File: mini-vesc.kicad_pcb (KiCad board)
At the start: 4 copper layers, 65 x 18 mm, 151 parts, among them P1 CONN_1, P10 CONN_01X06, P11 CONN_01X06, P2 CONN_1, P3 CONN_1, P4 CONN_1, P5 CONN_1, P6 CONN_1, P9 CONN_01X06, Q1 NTMFS5C604NLT1G, Q2 NTMFS5C604NLT1G, Q3 NTMFS5C604NLT1G, Q4 NTMFS5C604NLT1G, Q5 NTMFS5C604NLT1G, Q6 NTMFS5C604NLT1G, U1 LM5113, U10 MCP1700, U2 LM5113, U3 LM5113, U4 AD8418, U5 AD8418, U6 AD8418, U7 STM32F40X_LQFP64, U8 LMR16006, U9 MCP1700, X1 ABM3B-8.000MHZ

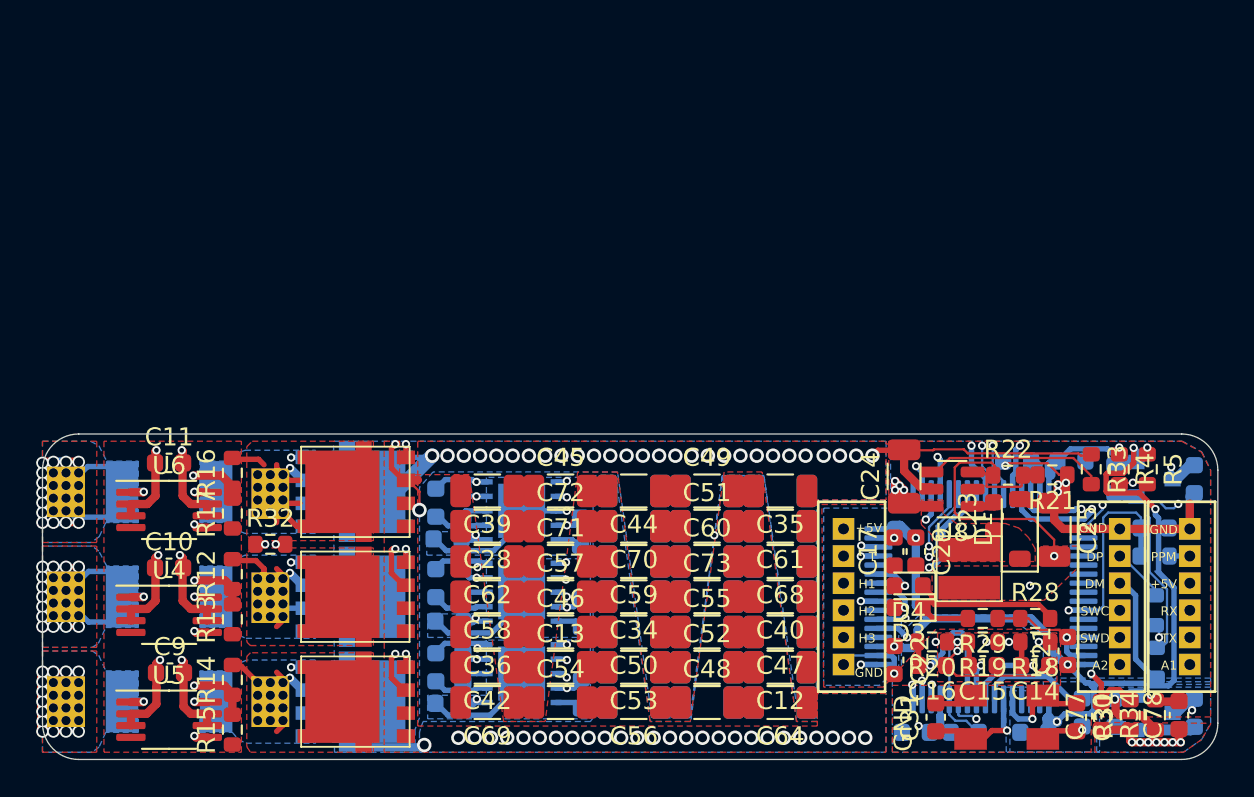
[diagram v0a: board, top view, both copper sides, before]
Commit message: Playing around with routing
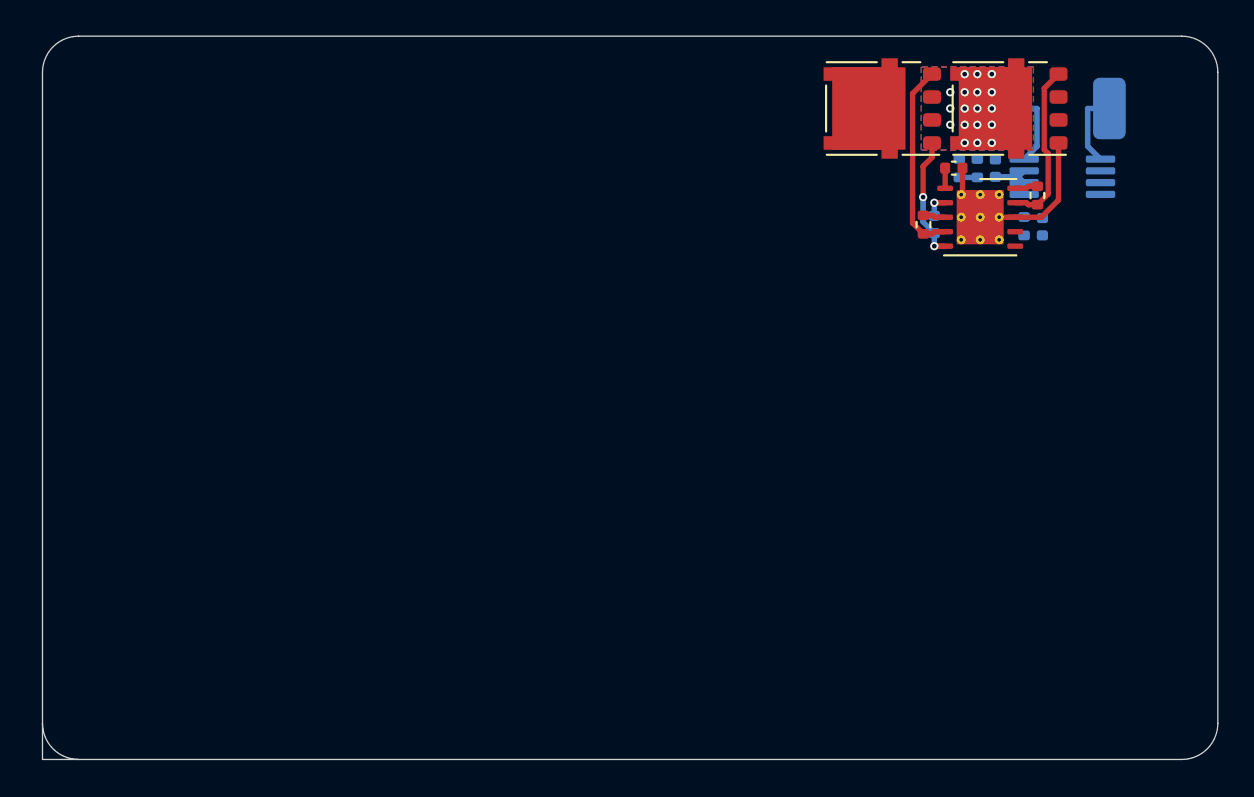
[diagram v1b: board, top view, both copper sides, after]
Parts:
- removed C1, C2, C3: 470n, Capacitor_SMD:C_0603_1608Metric
- removed C10, C11, C17, C18, C6, C7, C77, C78, C8, C86, C87, C88, C89, C9, C90: 2u2, Capacitor_SMD:C_0603_1608Metric
- removed C12, C13, C25, C28, C32, C39, C4, C48, C5, C60, C61, C62, C63, C74, C75, C84, C85: 10u, Capacitor_SMD:C_1206_3216Metric
- removed C14, C15, C16: 4n7, Capacitor_SMD:C_0603_1608Metric
- removed C19, C20, C21, C22, C26, C27, C29, C76: 100n, Capacitor_SMD:C_0603_1608Metric
- removed C23: 220nF, Capacitor_SMD:C_0603_1608Metric
- removed C24: 2u2, Capacitor_SMD:C_1206_3216Metric
- removed C30, C31: 10pF, Capacitor_SMD:C_0603_1608Metric
- removed C33, C34, C35, C36, C37, C38, C40, C41, C42, C43, C44, C45, C46, C47, C49, C50, C51, C52, C53, C54, C55, C56, C57, C58, C59, C64, C65, C66, C67, C68, C69, C70, C71, C72, C73, C83: C, Capacitor_SMD:C_1206_3216Metric
- removed D1: D_Schottky, Diode_SMD:D_SOD-123
- removed D3, D4: LED, LED_SMD:LED_0603_1608Metric
- removed L1: Wurth Electronics 74438335220, mojaKniznica:WE-MAPI
- removed P1, P2, P3, P4, P5, P6: CONN_1, kicad_subory:prekov
- removed P10, P11, P9: CONN_01X06, kicad_subory:JST_ZH_1.5_6-Pin
- removed Q1, Q2, Q5, Q6: NTMFS5C604NLT1G, kicad_subory:DFN5
- removed R1, R2, R3: R0005, mojaKniznica:2512Rv2
- removed R10, R11, R6, R7, R8, R9: 3R9, Resistor_SMD:R_0603_1608Metric
- removed R12, R14, R4: 39k, Resistor_SMD:R_0603_1608Metric
- removed R13, R15, R17, R5: 2k2, Resistor_SMD:R_0603_1608Metric
- removed R16: 25k5, Resistor_SMD:R_0603_1608Metric
- removed R18, R19, R20, R30: 100R, Resistor_SMD:R_0603_1608Metric
- removed R21, R31, R34: 10k, Resistor_SMD:R_0603_1608Metric
- removed R28, R29: 220R, Resistor_SMD:R_0603_1608Metric
- removed R32: 10kNTC, Resistor_SMD:R_0603_1608Metric
- removed R33: 100k, Resistor_SMD:R_0603_1608Metric
- removed U1, U2, U3: LM5113, kicad_subory:WSON10_
- removed U10, U9: MCP1700, TO_SOT_Packages_SMD:SOT-23
- removed U4: AD8418, Package_SO:MSOP-8_3x3mm_P0.65mm
- removed U7: STM32F40X_LQFP64, Package_QFP:LQFP-64_10x10mm_P0.5mm
- removed U8: LMR16006, Package_TO_SOT_SMD:SOT-23-6
- removed X1: ABM3B-8.000MHZ, mojaKniznica:5x3.2KRISTALL
- added R23: 3.9Ω, Resistor_SMD:R_0402_1005Metric, F.Cu at (123.0, 68.8)
- added R24: 39kΩ, Resistor_SMD:R_0402_1005Metric, B.Cu at (119.7, 67.3)
- added R26: 500µΩ, Footprints:R_Shunt_Bourns_CSS2H-2512_6332Metric, B.Cu at (124.4, 64.0)
- C79: value 10u -> 2.2µF; footprint Capacitor_SMD:C_1206_3216Metric -> Capacitor_SMD:C_0402_1005Metric; moved to F.Cu
- C80: value 10u -> 470nF; footprint Capacitor_SMD:C_1206_3216Metric -> Capacitor_SMD:C_0402_1005Metric
- C81: value C -> 2.2µF; footprint Capacitor_SMD:C_1206_3216Metric -> Capacitor_SMD:C_0402_1005Metric
- C82: value 10u -> 4.7nF; footprint Capacitor_SMD:C_1206_3216Metric -> Capacitor_SMD:C_0402_1005Metric
- Q3: footprint kicad_subory:DFN5 -> Package_SO:ONSemi_SO-8FL_488AA; moved to F.Cu
- Q4: footprint kicad_subory:DFN5 -> Package_SO:ONSemi_SO-8FL_488AA
- R22: value 54k9 -> 3.9Ω; footprint Resistor_SMD:R_0603_1608Metric -> Resistor_SMD:R_0402_1005Metric
- R25: value 22R -> 2.2kΩ; footprint Resistor_SMD:R_0603_1608Metric -> Resistor_SMD:R_0402_1005Metric
- R27: value 22R -> 100Ω; footprint Resistor_SMD:R_0603_1608Metric -> Resistor_SMD:R_0402_1005Metric
- U5: value AD8418 -> LM5113-Q1; footprint Package_SO:MSOP-8_3x3mm_P0.65mm -> Footprints:WSON-10-1EP_4x4mm_P0.8mm_EP2.6x3mm_ThermalVias
- U6: value AD8418 -> AD8417; moved to B.Cu
- moved U5 52.8 mm to (119.9, 70.0)
- moved U6 52.7 mm to (124.4, 67.8), turned to 180 degrees
- moved Q4 48.8 mm to (121.4, 64.0)
- moved Q3 43.9 mm to (114.4, 64.0), turned to 180 degrees
- moved C81 30.1 mm to (120.7, 67.3), turned to -90 degrees
- moved C82 30.0 mm to (123.3, 70.5), turned to -90 degrees
- moved R25 29.4 mm to (118.7, 67.3), turned to -90 degrees
- moved R27 22.4 mm to (122.3, 70.5)
- moved C79 20.3 mm to (118.4, 67.3), turned to 0 degrees
- moved C80 18.7 mm to (117.3, 70.4), turned to -90 degrees
- moved R22 14.6 mm to (116.7, 70.4), turned to 90 degrees
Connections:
- C79 pad 1: VDD -> +5V
- C80 pad 1: VDD -> Net-(U5-HB)
- C80 pad 2: VSS -> /Half Bridge W/Output
- C81 pad 1: VDD -> VSS
- C81 pad 2: VSS -> VAA
- C82 pad 1: VDD -> VSS
- C82 pad 2: VSS -> I_{senseW}
- Q3 pad 1: Net-(Q3-G) -> /Half Bridge W/Output
- Q3 pad 2: SH2 -> /Half Bridge W/Output
- Q3 pad 3: VDD -> /Half Bridge W/Output
- Q4 pad 1: Net-(Q4-G) -> VSS
- Q4 pad 3: SH2 -> VSS
- R22 pad 1: +5V -> /Half Bridge W/HighGate
- R22 pad 2: Net-(U8-FB) -> Net-(U5-HOH)
- R25 pad 1: Net-(P10-Pin_4) -> VSS
- R25 pad 2: USB-DM -> V_{senseW}
- R27 pad 1: Net-(P10-Pin_5) -> Net-(U6-OUT)
- R27 pad 2: USB-DP -> I_{senseW}
- U5 pad 1: Net-(P2-Pad1) -> +5V
- U5 pad 2: VSS -> Net-(U5-HB)
- U5 pad 3: VSS -> Net-(U5-HOH)
- U5 pad 4: Net-(U5-Pad4) -> /Half Bridge W/HighGate
- U5 pad 5: I2 -> /Half Bridge W/Output
- U5 pad 6: VAA -> HI3
- U5 pad 7: VAA -> LI3
- U5 pad 8: SH2 -> VSS
- U6 pad 1: Net-(P3-Pad1) -> /W
- U6 pad 4: Net-(U6-Pad4) -> unconnected-(U6-NC-Pad4)
- U6 pad 5: I3 -> Net-(U6-OUT)
- U6 pad 8: SH3 -> /Half Bridge W/Output
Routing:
- net VSS: track 298.6 -> 8.32 mm, vias 57 -> 0
- net +5V: track 162.2 -> 1.11 mm, vias 6 -> 0
- net VAA: track 134.2 -> 3.44 mm, vias 6 -> 0
- net VDD: track 93.0 -> 0.00 mm, vias 30 -> 0
- net VCC: track 82.9 -> 0.00 mm, vias 6 -> 0
- net Net-(C77-Pad2): track 67.6 -> 0.00 mm
- net I1: track 60.9 -> 0.00 mm, vias 2 -> 0
- net I3: track 60.2 -> 0.00 mm, vias 2 -> 0
- net SENS_3: track 53.9 -> 0.00 mm, vias 2 -> 0
- net SENS_2: track 51.4 -> 0.00 mm, vias 2 -> 0
- net SENS_1: track 49.8 -> 0.00 mm, vias 2 -> 0
- net I2: track 48.2 -> 0.00 mm, vias 2 -> 0
- net ADC_EXT1: track 41.7 -> 0.00 mm, vias 3 -> 0
- net HI2: track 31.2 -> 0.00 mm, vias 2 -> 0
- net TX: track 29.4 -> 0.00 mm, vias 1 -> 0
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- added copper zone on B.Cu, net /Half Bridge W/Output
- added copper zone on F.Cu, net /Half Bridge W/Output
- removed copper zone on F.Cu, net +5V
- removed copper zone on F.Cu, net Net-(D1-K)
- removed copper zone on B.Cu, net Net-(U4-IN-)
- removed copper zone on F.Cu, net Net-(U4-IN-)
- removed copper zone on In1.Cu, net Net-(U4-IN-)
- removed copper zone on In2.Cu, net Net-(U4-IN-)
- removed copper zone on B.Cu, net Net-(U5-IN-)
- removed copper zone on F.Cu, net Net-(U5-IN-)
- removed copper zone on In1.Cu, net Net-(U5-IN-)
- removed copper zone on In2.Cu, net Net-(U5-IN-)
- removed copper zone on B.Cu, net Net-(U6-IN-)
- removed copper zone on F.Cu, net Net-(U6-IN-)
- removed copper zone on In1.Cu, net Net-(U6-IN-)
- removed copper zone on In2.Cu, net Net-(U6-IN-)
- removed copper zone on B.Cu, net SH1
- removed copper zone on F.Cu, net SH1
- removed copper zone on B.Cu, net SH2
- removed copper zone on F.Cu, net SH2
- removed copper zone on B.Cu, net SH3
- removed copper zone on F.Cu, net SH3
- removed copper zone on B.Cu, net VDD
- removed copper zone on F.Cu, net VDD
- removed copper zone on In1.Cu, net VDD
- removed copper zone on In2.Cu, net VDD
- removed copper zone on B.Cu, net VSS
- removed copper zone on F.Cu, net VSS
- removed copper zone on In1.Cu, net VSS
- removed copper zone on In2.Cu, net VSS
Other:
- board size 65 x 18 mm -> 65 x 40 mm
- board text removed: "+5V"
- board text removed: "A1"
- board text removed: "A2"
- board text removed: "DM"
- board text removed: "DP"
- board text removed: "GND"
- board text removed: "H1"
- board text removed: "H2"
- board text removed: "H3"
- board text removed: "PPM"
- board text removed: "RX"
- board text removed: "SWC"
- board text removed: "SWD"
- board text removed: "T"
- board text removed: "TX"
